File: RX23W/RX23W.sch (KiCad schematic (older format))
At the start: 2 parts

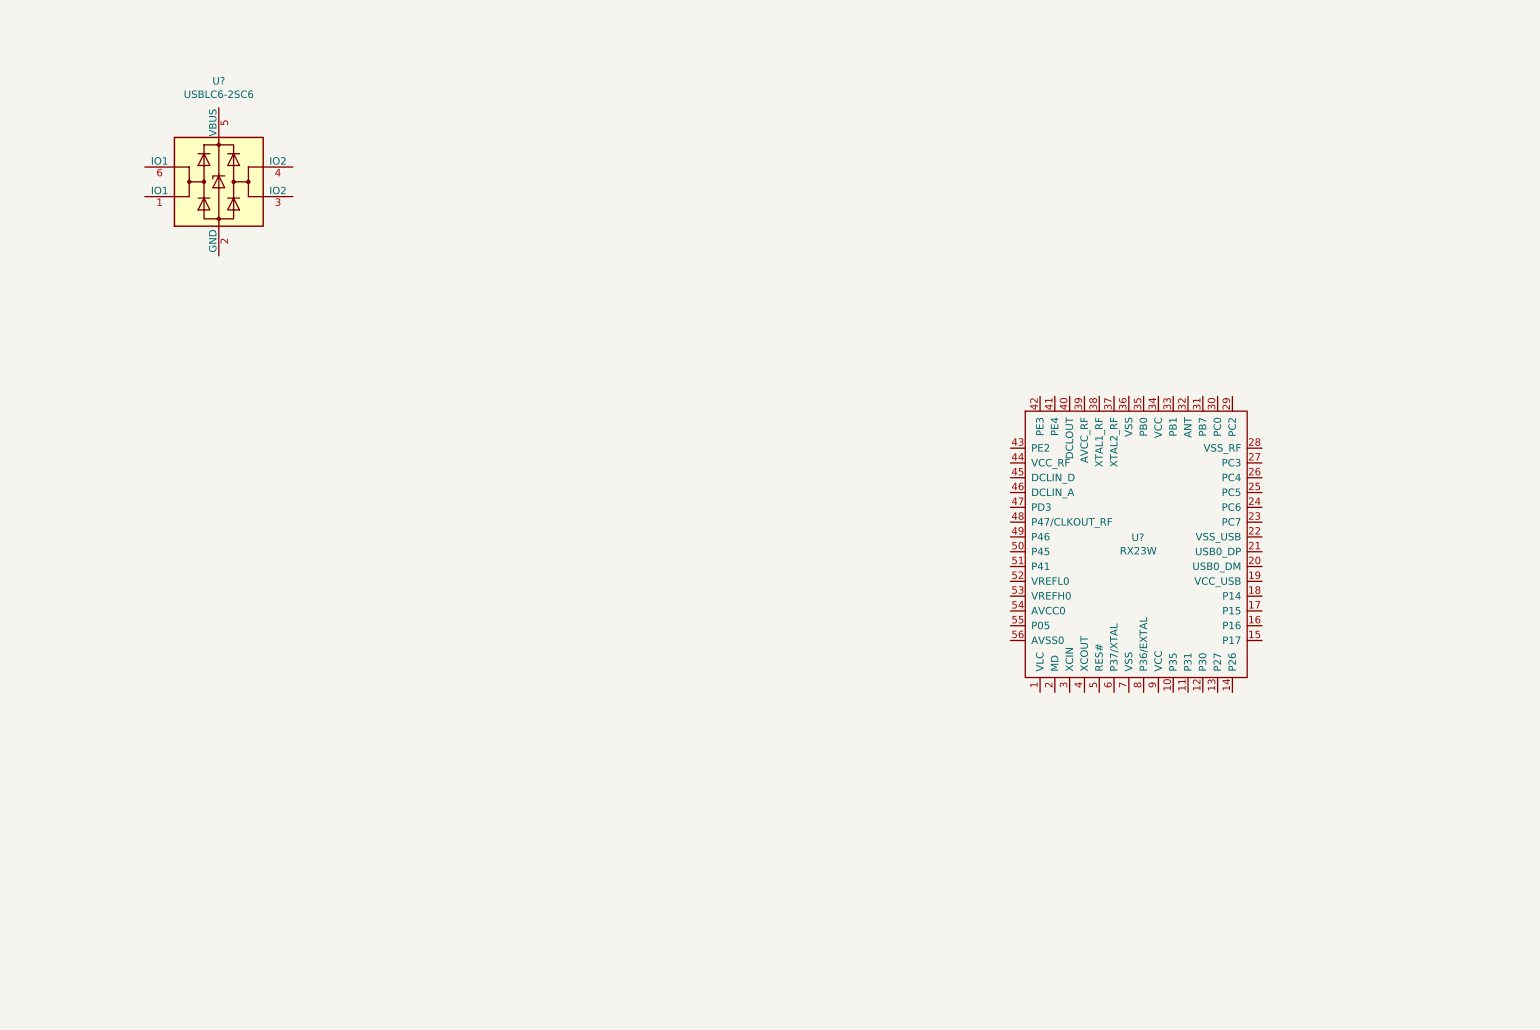
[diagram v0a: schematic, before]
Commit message: Schematics
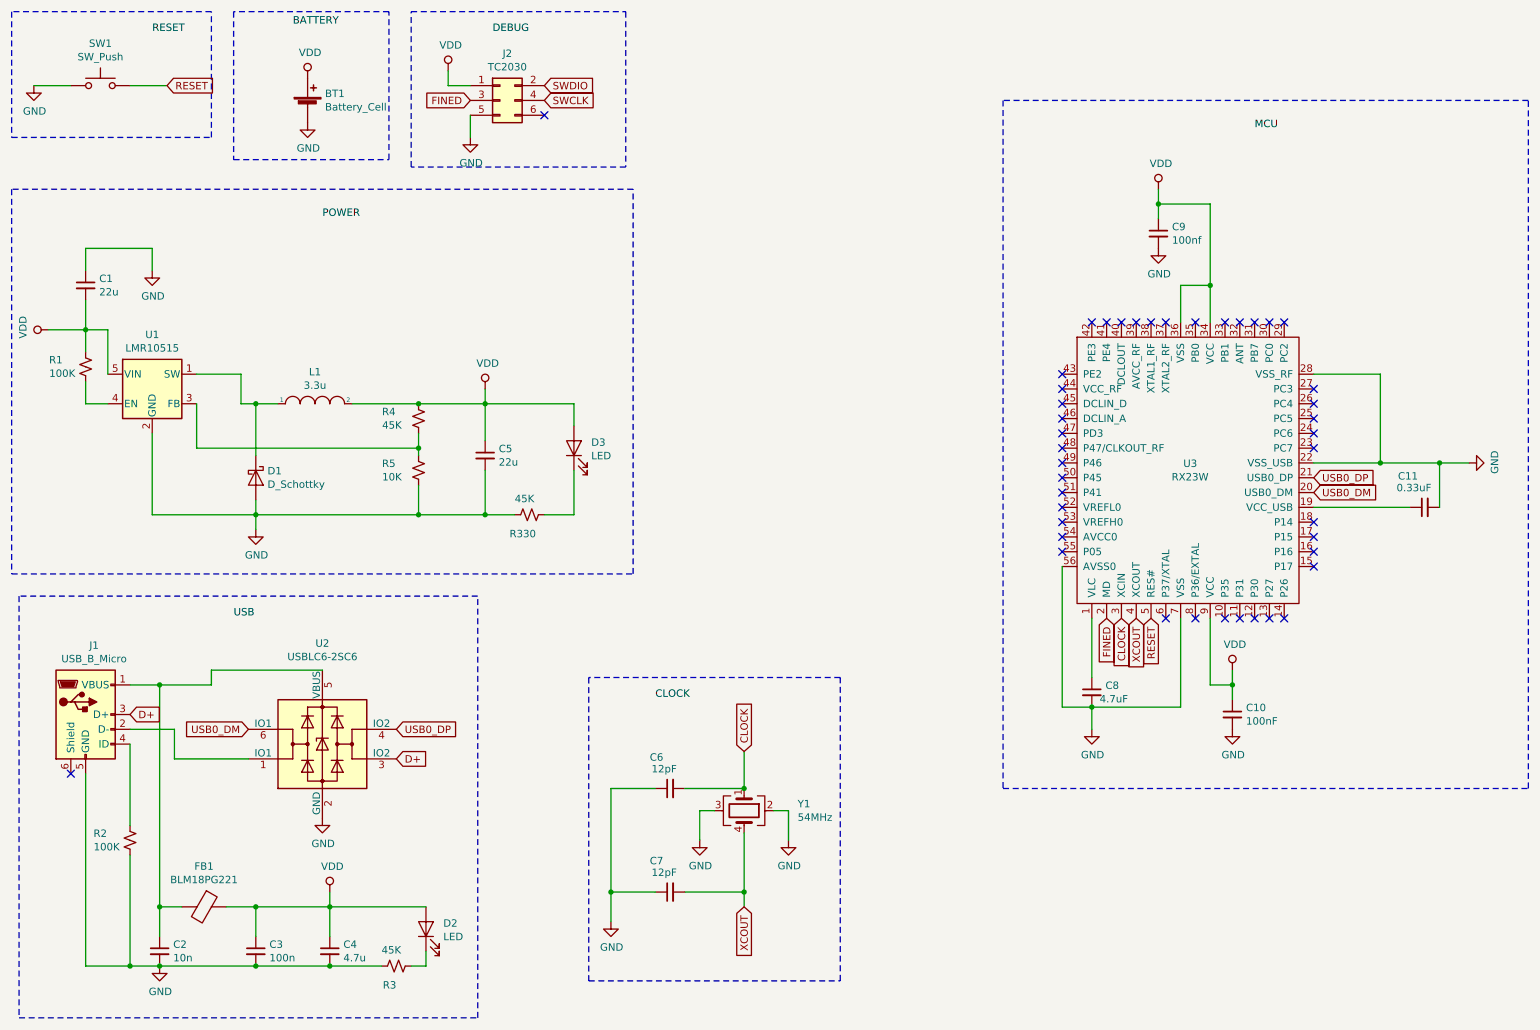
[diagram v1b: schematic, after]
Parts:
- added BT1: Battery_Cell, symbol Device:Battery_Cell
- added C1, C5: 22u, symbol Device:C_Small
- added C10: 100nF, symbol Device:C_Small
- added C11: 0.33uF, symbol Device:C_Small
- added C2: 10n, symbol Device:C_Small
- added C3: 100n, symbol Device:C_Small
- added C4: 4.7u, symbol Device:C_Small
- added C6, C7: 12pF, symbol Device:C_Small
- added C8: 4.7uF, symbol Device:C_Small
- added C9: 100nf, symbol Device:C_Small
- added D1: D_Schottky, symbol Device:D_Schottky
- added D2, D3: LED, symbol Device:LED
- added FB1: BLM18PG221, symbol Device:Ferrite_Bead
- added J1: USB_B_Micro, symbol Connector:USB_B_Micro
- added J2: TC2030, symbol Connector_Generic:Conn_02x03_Odd_Even
- added L1: 3.3u, symbol pspice:INDUCTOR
- added R1, R2: 100K, symbol Device:R_Small_US
- added R3, R330, R4: 45K, symbol Device:R_Small_US
- added R5: 10K, symbol Device:R_Small_US
- added SW1: SW_Push, symbol Switch:SW_Push
- added U1: LMR10515, Package_TO_SOT_SMD:SOT-23-5, symbol Regulator_Switching:LMR10510XMF
- added Y1: 54MHz, symbol Device:Crystal_GND23
- gave numbers to parts that had none: 2
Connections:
- net at U3.1 (VLC): now also C8.1
- net at U3.19 (VCC_USB): now also C11.1
- net FINED: now reaches U3.2 (MD)
- net FINED: now also J2.3 (Pin_3)
- net USB0_DM: now reaches U3.20 (USB0_DM)
- net USB0_DM: now also U2.6 (IO1)
- net USB0_DP: now reaches U3.21 (USB0_DP)
- net USB0_DP: now also U2.4 (IO2)
- net GND: now reaches U3.22 (VSS_USB)
- net GND: now also U2.2 (GND), U3.28 (VSS_RF), U3.56 (AVSS0), U3.7 (VSS), BT1.2 (-), C1.1, C10.2, C11.2, C2.2, C3.2, C4.2, C5.2, C6.1, C7.1, C8.2, C9.2, D1.2 (A), J1.5 (GND), J2.5 (Pin_5), R2.2, R3.1, R330.1, R5.2, SW1.1, U1.2 (GND), Y1.2, Y1.3
- net CLOCK: now reaches U3.3 (XCIN)
- net CLOCK: now also C6.2, Y1.1
- net VDD: now reaches U3.34 (VCC)
- net VDD: now also U3.36 (VSS), U3.9 (VCC), BT1.1 (+), C1.2, C10.1, C3.1, C4.1, C5.1, C9.1, D2.2 (A), D3.2 (A), FB1.1, J2.1 (Pin_1), L1.2, R1.1, R4.1, U1.5 (VIN)
- net XCOUT: now reaches U3.4 (XCOUT)
- net XCOUT: now also C7.2, Y1.4
- net RESET: now reaches U3.5 (RES#)
- net RESET: now also SW1.2
- net at U2.1 (IO1): now also J1.2 (D-)
- net D+: now reaches U2.3 (IO2)
- net D+: now also J1.3 (D+)
- net at U2.5 (VBUS): now also C2.1, FB1.2, J1.1 (VBUS)
- new net: J1.4 (ID), R2.1
- new net: D1.1 (K), L1.1, U1.1 (SW)
- new net: R4.2, R5.1, U1.3 (FB)
- new net: R1.2, U1.4 (EN)
- new net: D3.1 (K), R330.2
- new net: D2.1 (K), R3.2
- new net SWCLK: J2.4 (Pin_4)
- new net SWDIO: J2.2 (Pin_2)
- no-connect marks 0 -> 43
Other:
- moved on the sheet: U2, U3

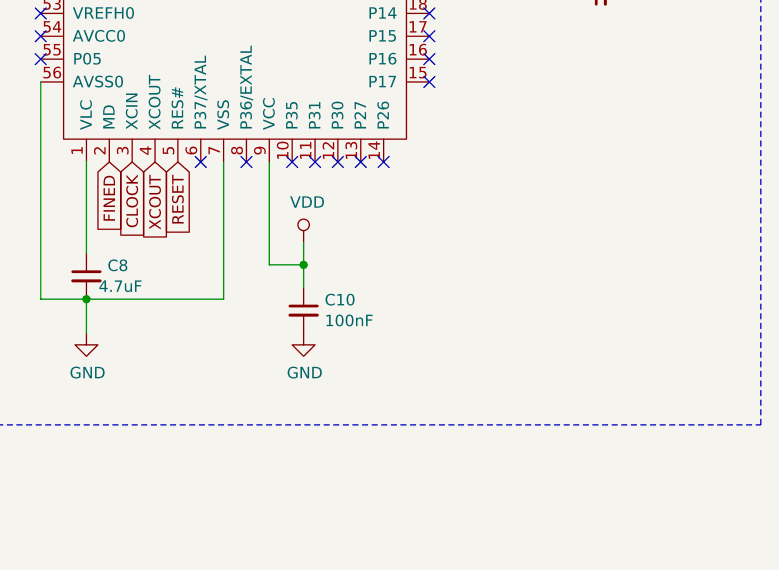
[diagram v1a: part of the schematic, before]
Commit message: Altered
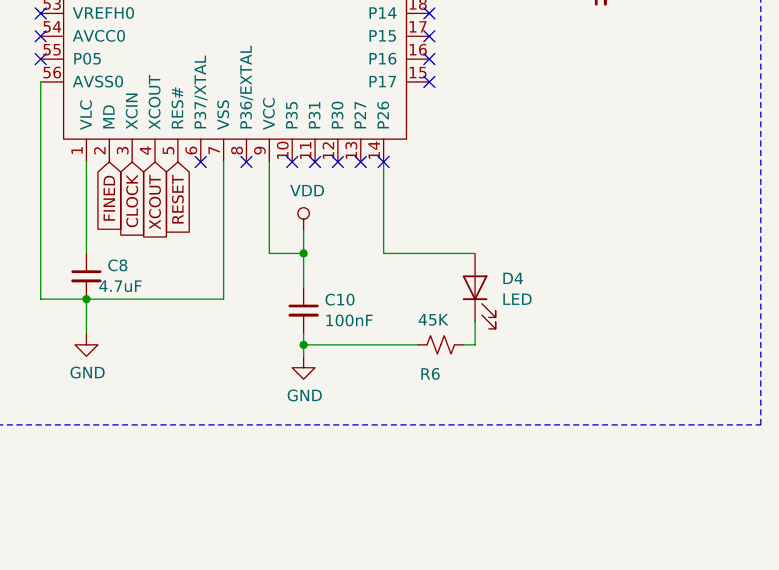
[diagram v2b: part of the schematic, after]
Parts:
- added D4: LED, symbol Device:LED
- added R6: 45K, symbol Device:R_Small_US
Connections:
- net GND: now also R6.1
- net at U3.14 (P26): now also D4.2 (A)
- new net: D4.1 (K), R6.2
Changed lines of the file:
@@
 $EndDescr
-$Comp
-L RX23W:RX23W U3
-U 1 1 5DFAF628
-P 8150 4450
-F 0 "U3" H 8618 5096 50  0000 L CNN
-F 1 "RX23W" H 8539 5005 50  0000 L CNN
-F 2 "" H 8600 5050 50  0001 C CNN
-F 3 "" H 8600 5050 50  0001 C CNN
-	1    8150 4450
-	1    0    0    -1
-$EndComp
 $Comp
 L power:GND #PWR08
@@
 L power:GND #PWR020
 U 1 1 5DFF9F75
-P 8950 5600
-F 0 "#PWR020" H 8950 5350 50  0001 C CNN
-F 1 "GND" H 8955 5427 50  0000 C CNN
-F 2 "" H 8950 5600 50  0001 C CNN
-F 3 "" H 8950 5600 50  0001 C CNN
-	1    8950 5600
+P 8950 5700
+F 0 "#PWR020" H 8950 5450 50  0001 C CNN
+F 1 "GND" H 8955 5527 50  0000 C CNN
+F 2 "" H 8950 5700 50  0001 C CNN
+F 3 "" H 8950 5700 50  0001 C CNN
+	1    8950 5700
 	1    0    0    -1
 $EndComp
@@
 L power:VDD #PWR019
 U 1 1 5DFFA7AD
-P 8950 5200
-F 0 "#PWR019" H 8950 5050 50  0001 C CNN
-F 1 "VDD" H 8967 5373 50  0000 C CNN
-F 2 "" H 8950 5200 50  0001 C CNN
-F 3 "" H 8950 5200 50  0001 C CNN
-	1    8950 5200
-	1    0    0    -1
-$EndComp
-Wire Wire Line
-	8800 4850 8800 5300
+P 8950 5150
+F 0 "#PWR019" H 8950 5000 50  0001 C CNN
+F 1 "VDD" H 8967 5323 50  0000 C CNN
+F 2 "" H 8950 5150 50  0001 C CNN
+F 3 "" H 8950 5150 50  0001 C CNN
+	1    8950 5150
+	1    0    0    -1
+$EndComp
 $Comp
 L Device:C_Small C9
@@
 NoConn ~ 9000 4850
 NoConn ~ 9100 4850
-NoConn ~ 9200 4850
-NoConn ~ 9300 4850
-Wire Wire Line
-	8950 5200 8950 5300
-Wire Wire Line
-	8800 5300 8950 5300
-Connection ~ 8950 5300
-Wire Wire Line
-	8950 5300 8950 5400
 Wire Notes Line
 	10950 6000 10950 1350
@@
 NoConn ~ 7800 4300
 NoConn ~ 7800 4400
+$Comp
+L Device:LED D4
+U 1 1 5E2482DA
+P 9700 5400
+F 0 "D4" V 9739 5283 50  0000 R CNN
+F 1 "LED" V 9648 5283 50  0000 R CNN
+F 2 "" H 9700 5400 50  0001 C CNN
+F 3 "~" H 9700 5400 50  0001 C CNN
+	1    9700 5400
+	0    -1   -1   0
+$EndComp
+$Comp
+L Device:R_Small_US R6
+U 1 1 5E2482E0
+P 9550 5650
+F 0 "R6" V 9421 5696 50  0000 C CNN
+F 1 "45K" V 9658 5684 50  0000 C CNN
+F 2 "" H 9550 5650 50  0001 C CNN
+F 3 "~" H 9550 5650 50  0001 C CNN
+	1    9550 5650
+	0    -1   -1   0
+$EndComp
+Wire Wire Line
+	9650 5650 9700 5650
+Wire Wire Line
+	9700 5650 9700 5550
+Wire Wire Line
+	8950 5600 8950 5650
+Wire Wire Line
+	9450 5650 8950 5650
+Connection ~ 8950 5650
+Wire Wire Line
+	8950 5650 8950 5700
+Wire Wire Line
+	8800 4850 8800 5250
+Wire Wire Line
+	8800 5250 8950 5250
+Connection ~ 8950 5250
+Wire Wire Line
+	8950 5250 8950 5400
+Wire Wire Line
+	8950 5150 8950 5250
+Wire Wire Line
+	9700 5250 9300 5250
+Wire Wire Line
+	9300 5250 9300 4850
+NoConn ~ 9300 4850
+$Comp
+L RX23W:RX23W U3
+U 1 1 5DFAF628
+P 8150 4450
+F 0 "U3" H 8618 5096 50  0000 L CNN
+F 1 "RX23W" H 8539 5005 50  0000 L CNN
+F 2 "" H 8600 5050 50  0001 C CNN
+F 3 "" H 8600 5050 50  0001 C CNN
+	1    8150 4450
+	1    0    0    -1
+$EndComp
+NoConn ~ 9200 4850
 $EndSCHEMATC
